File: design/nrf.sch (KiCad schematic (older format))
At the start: 17 parts, among them U8 NRF24L01P, U9 CONN_U_FL, X2 16M

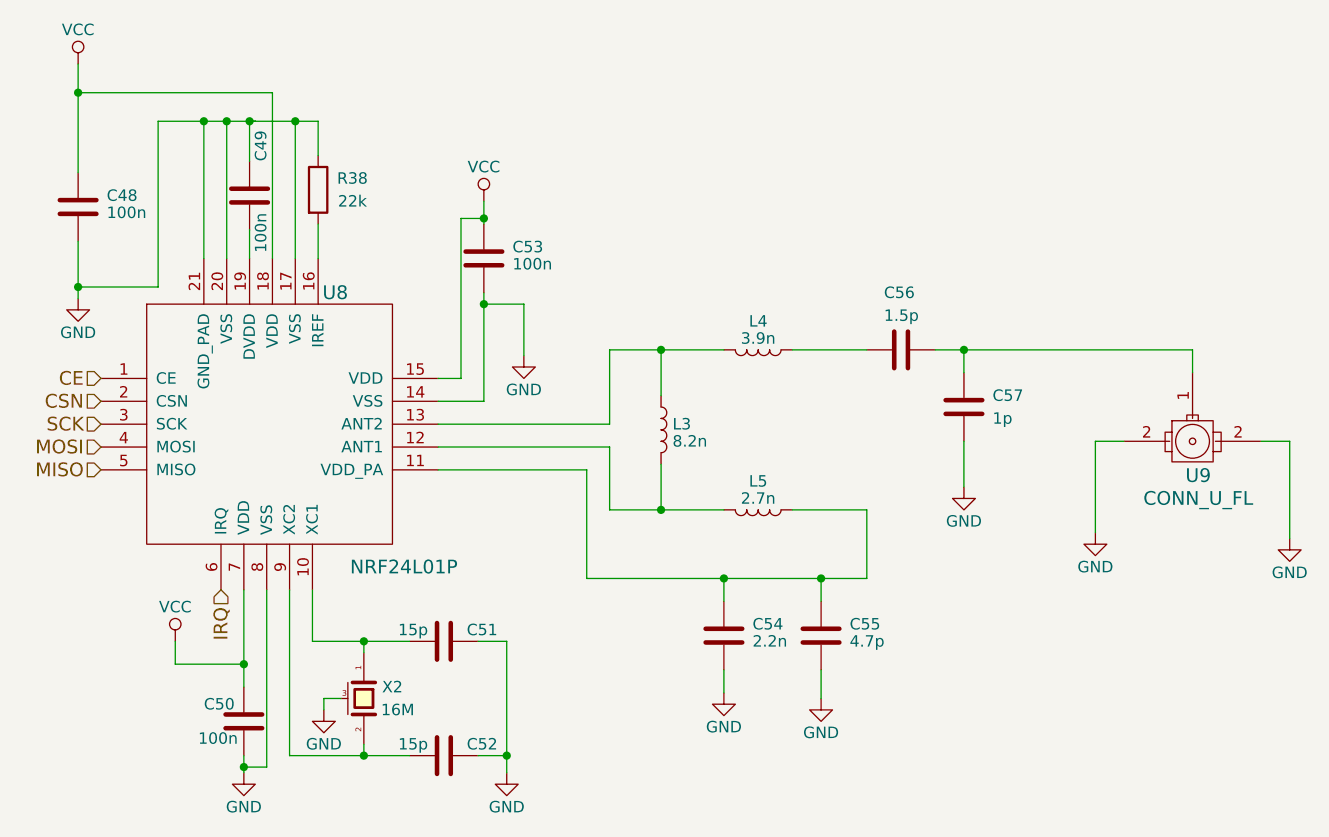
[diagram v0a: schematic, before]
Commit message: initial commit
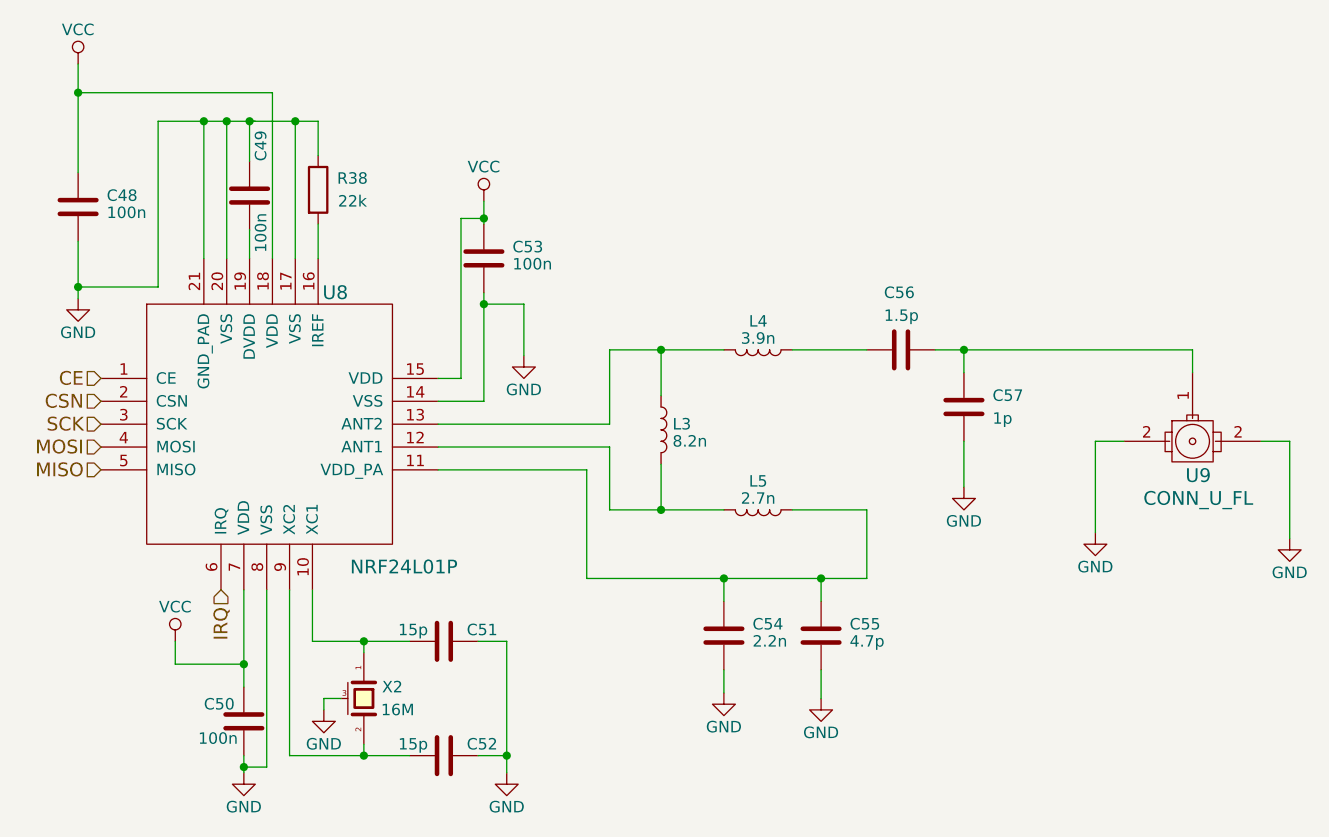
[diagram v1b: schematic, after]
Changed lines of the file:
@@
 	4200 4400 4200 5175
 Wire Wire Line
-	4100 4400 4100 4725
-Wire Wire Line
-	4100 4725 4100 4825
+	4100 4400 4100 4825
 Wire Wire Line
 	4400 4400 4400 4625
 Wire Wire Line
-	4400 4625 4625 4625
-Wire Wire Line
-	4625 4625 4825 4625
+	4400 4625 4825 4625
 Connection ~ 4625 4625
 Wire Wire Line
@@
 	5125 4625 5250 4625
 Wire Wire Line
-	5250 4625 5250 5125
-Wire Wire Line
-	5250 5125 5250 5200
+	5250 4625 5250 5200
 Wire Wire Line
 	4625 5075 4625 5125
@@
 Connection ~ 5250 5125
 Wire Wire Line
-	4300 5125 4625 5125
-Wire Wire Line
-	4625 5125 4825 5125
+	4300 5125 4825 5125
 Wire Wire Line
 	5125 5125 5250 5125
@@
 	5700 3675 5700 3350
 Wire Wire Line
-	5700 3350 5925 3350
-Wire Wire Line
-	5925 3350 6200 3350
+	5700 3350 6200 3350
 Wire Wire Line
 	4950 3875 5600 3875
@@
 	5600 3875 5600 4350
 Wire Wire Line
-	5600 4350 6200 4350
-Wire Wire Line
-	6200 4350 6625 4350
-Wire Wire Line
-	6625 4350 6825 4350
+	5600 4350 6825 4350
 Wire Wire Line
 	6825 4350 6825 4050
@@
 	4325 2350 4325 2950
 Wire Wire Line
-	3725 2350 3925 2350
-Wire Wire Line
-	3925 2350 4025 2350
-Wire Wire Line
-	4025 2350 4125 2350
-Wire Wire Line
-	4325 2350 4425 2350
+	3725 2350 4425 2350
 Wire Wire Line
 	3725 3075 3725 2350
@@
 Connection ~ 3925 2350
 Wire Wire Line
-	4100 5125 4100 5175
-Wire Wire Line
-	4100 5175 4100 5200
+	4100 5125 4100 5200
 Wire Wire Line
 	4200 5175 4100 5175
 Connection ~ 4100 5175
 Wire Wire Line
-	5150 2700 5150 2775
+	5150 2700 5150 2800
 Wire Wire Line
-	5150 2775 5150 2800
-Wire Wire Line
-	5150 3100 5150 3150
-Wire Wire Line
-	5150 3150 5150 3575
+	5150 3100 5150 3575
 Connection ~ 5150 3150
 Wire Wire Line
@@
 Connection ~ 5150 2775
 Wire Wire Line
-	3375 2100 3375 2225
+	3375 2100 3375 2575
 Wire Wire Line
-	3375 2225 3375 2575
-Wire Wire Line
-	3375 2875 3375 3075
-Wire Wire Line
-	3375 3075 3375 3125
+	3375 2875 3375 3125
 Connection ~ 3375 3075
 Wire Wire Line
 	4125 2825 4125 2950
 Wire Wire Line
-	4125 2525 4125 2350
+	4125 2350 4125 2525
 Wire Wire Line
 	6825 3350 6500 3350
@@
 	5325 3150 5325 3375
 Wire Wire Line
-	5700 4050 5925 4050
-Wire Wire Line
-	5925 4050 6200 4050
+	5700 4050 6200 4050
 Wire Wire Line
 	5925 3850 5925 4050
@@
 Connection ~ 7250 3350
 Wire Wire Line
-	7125 3350 7250 3350
-Wire Wire Line
-	7250 3350 8250 3350
+	7125 3350 8250 3350
 Wire Wire Line
 	8250 3350 8250 3450
@@
 Wire Wire Line
 	4125 2350 4150 2350
-Wire Wire Line
-	4150 2350 4325 2350
-Wire Wire Line
-	4125 2350 4150 2350

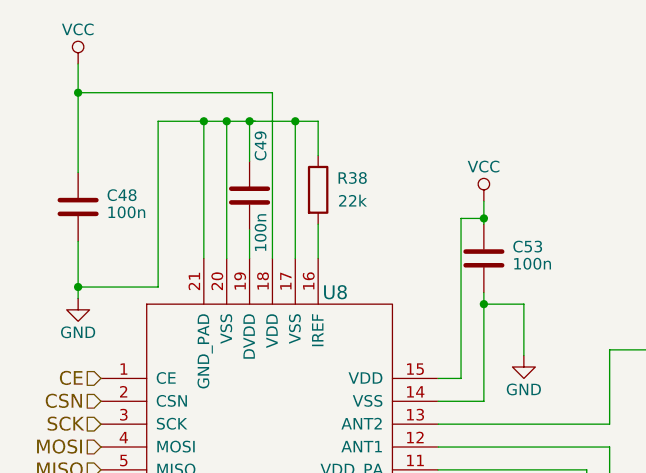
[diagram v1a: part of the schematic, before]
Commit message: initial commit
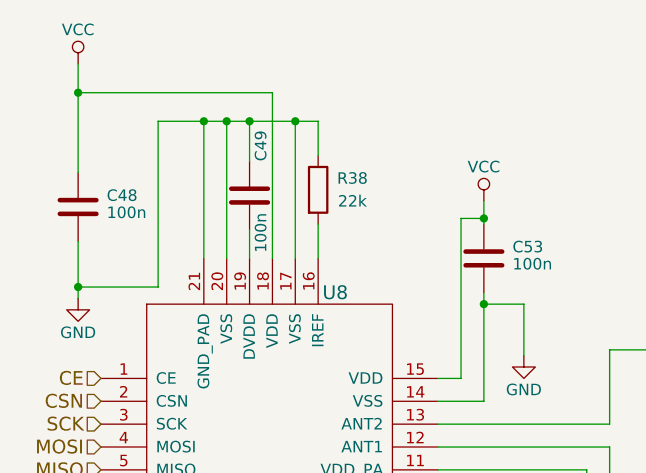
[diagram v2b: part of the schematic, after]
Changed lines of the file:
@@
 LIBS:valves
 LIBS:crf_1
-LIBS:VESC_6-cache
 EELAYER 25 0
 EELAYER END
@@
 	4325 2350 4325 2950
 Wire Wire Line
-	3725 2350 4425 2350
-Wire Wire Line
 	3725 3075 3725 2350
 Wire Wire Line
@@
 Connection ~ 3375 2225
 Wire Wire Line
-	4025 2950 4025 2350
+	4025 2350 4025 2950
 Connection ~ 4025 2350
 Wire Wire Line
@@
 Wire Wire Line
 	4425 2800 4425 2950
-Connection ~ 4325 2350
-Connection ~ 4125 2350
 Wire Wire Line
 	3925 2950 3925 2350
@@
 	4450 4875 4450 4925
 Wire Wire Line
-	4125 2350 4150 2350
+	3725 2350 4425 2350
+Connection ~ 4125 2350
+Connection ~ 4325 2350
 $EndSCHEMATC
